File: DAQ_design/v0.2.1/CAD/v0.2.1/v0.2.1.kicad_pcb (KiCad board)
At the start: 2 copper layers, 119 x 75 mm, 36 parts, among them J1 Screw_Terminal_01x04, U1 Teensy4.0, U2 L293D, U3 PC817, U5 PC817, U6 PC817, U7 74HC165

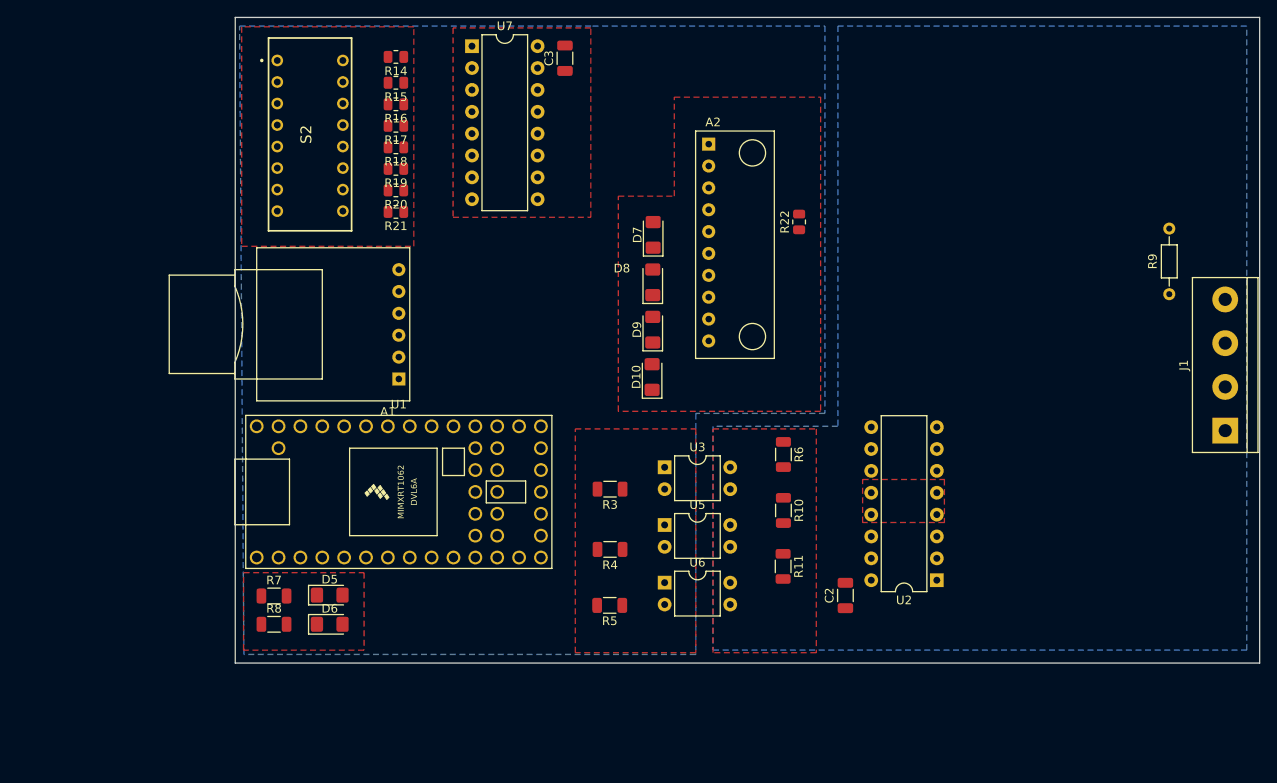
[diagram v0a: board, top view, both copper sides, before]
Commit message: resync
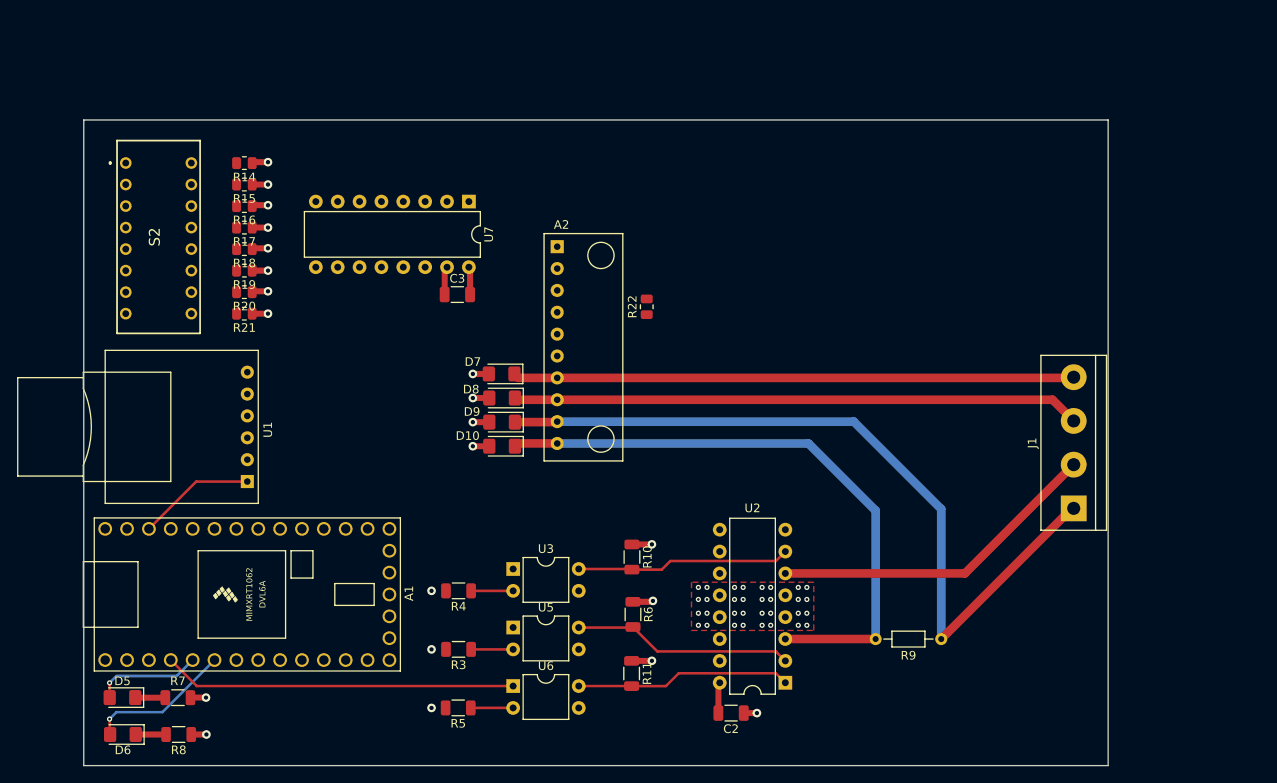
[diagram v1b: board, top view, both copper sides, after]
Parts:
- moved R9 48.0 mm to (185.0, 123.7), turned to 180 degrees
- moved C3 30.2 mm to (128.8, 83.7), turned to 0 degrees
- moved D6 27.2 mm to (90.0, 134.8), turned to 180 degrees
- moved D5 26.9 mm to (89.9, 130.5), turned to 180 degrees
- moved R3 25.6 mm to (128.9, 124.9)
- moved R6 25.5 mm to (149.2, 120.8)
- moved D7 23.9 mm to (133.9, 92.9), turned to 180 degrees
- moved D8 22.1 mm to (134.0, 95.7), turned to 180 degrees
- moved R11 21.6 mm to (149.0, 127.7)
- moved R14 21.5 mm to (104.1, 68.4)
- moved U6 21.3 mm to (135.3, 129.2)
- moved R5 21.3 mm to (128.9, 131.7)
- moved U5 21.3 mm to (135.3, 122.4)
- moved A1 21.3 mm to (104.4, 105.4)
- moved A2 21.3 mm to (140.4, 78.1)
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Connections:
- A2 pad 10: IN3 -> EX+
- A2 pad 7: EX+ -> IN2
- A2 pad 8: IN1 -> IN3
- A2 pad 9: IN2 -> IN1
- D10 pad 1: IN3 -> EX+
- D7 pad 1: EX+ -> IN2
- D8 pad 1: IN1 -> IN3
- D9 pad 1: IN2 -> IN1
- J1 pad 1: IN2 -> IN1
- J1 pad 2: IN3 -> EX-
- J1 pad 3: EX- -> IN3
- J1 pad 4: IN1 -> IN2
- U1 pad 16: +3.3V -> unconnected-(U1-3V3-Pad16)
- U1 pad 23: unconnected-(U1-16_A2_RX4_SCL1-Pad23) -> ADC_SCL
- U1 pad 24: unconnected-(U1-17_A3_TX4_SDA1-Pad24) -> ADC_SDA
- U1 pad 25: ADC_SDA -> unconnected-(U1-18_A4_SDA0-Pad25)
- U1 pad 26: ADC_SCL -> unconnected-(U1-19_A5_SCL0-Pad26)
- U3 pad 1: LOGIC1 -> LOGIC2
- U3 pad 2: Net-(R3-Pad1) -> Net-(R4-Pad1)
- U3 pad 4: OPT1 -> OPT2
- U5 pad 1: LOGIC2 -> LOGIC1
- U5 pad 2: Net-(R4-Pad1) -> Net-(R3-Pad1)
- U5 pad 4: OPT2 -> OPT1
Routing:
- net IN1: track 0.00 -> 90.5 mm
- net EX+: track 0.00 -> 70.7 mm
- net IN3: track 0.00 -> 66.0 mm
- net IN2: track 0.00 -> 65.2 mm
- net EN: track 0.00 -> 41.0 mm
- net EX-: track 0.00 -> 38.7 mm
- net GNDD: track 0.00 -> 29.2 mm, vias 0 -> 17
- net OPT1: track 0.00 -> 25.7 mm
- net OPTEN: track 0.00 -> 25.1 mm
- net OPT2: track 0.00 -> 24.9 mm
- net LEDACT: track 0.00 -> 16.9 mm, vias 0 -> 1
- net +3.3V: track 0.00 -> 13.7 mm
- net LEDPOW: track 0.00 -> 12.5 mm, vias 0 -> 1
- net VPP: track 0.00 -> 10.6 mm, vias 0 -> 3
- net Net-(R5-Pad1): track 0.00 -> 4.92 mm
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- added copper zone on In1.Cu, net GND
- added copper zone on In1.Cu, net GNDD
- added copper zone on In2.Cu, net VDD
- added copper zone on In2.Cu, net VPP
- removed copper zone on B.Cu, net GND
- removed copper zone on B.Cu, net GNDD
- removed copper zone on F.Cu, net GNDD
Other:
- copper layers 2 -> 4
